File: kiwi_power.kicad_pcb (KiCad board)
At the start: 2 copper layers, 100 x 92 mm, 60 parts, among them J1 PSU, J10 Power_output, J2 Battery, J3 emergency_stop, J4 Power_always, J5 Power_stop, J6 Power_output, J7 Power_output, J8 Power_output, J9 Power_output, K1 SANYOU_SRD_Form_C, Q1 BC327, Q2 IRF9540N, Q3 BC327, Q4 BC327, Q5 IRF9540N, Q6 BC327, U1 LM317_TO-220, U2 lm2596_blue_board, U3 lm2596_blue_board, U4 lm2596_blue_board, U5 lm2596_blue_board, U6 lm2596_blue_board

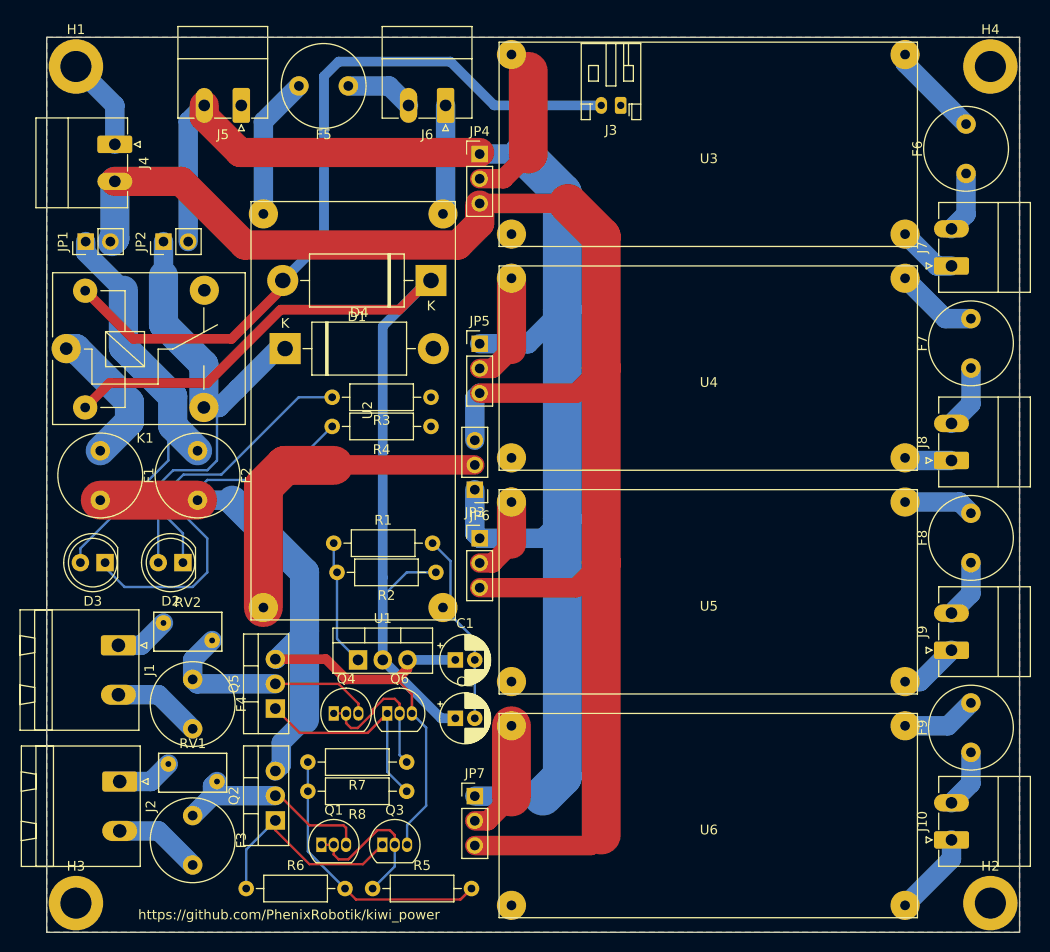
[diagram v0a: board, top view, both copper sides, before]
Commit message: version 2
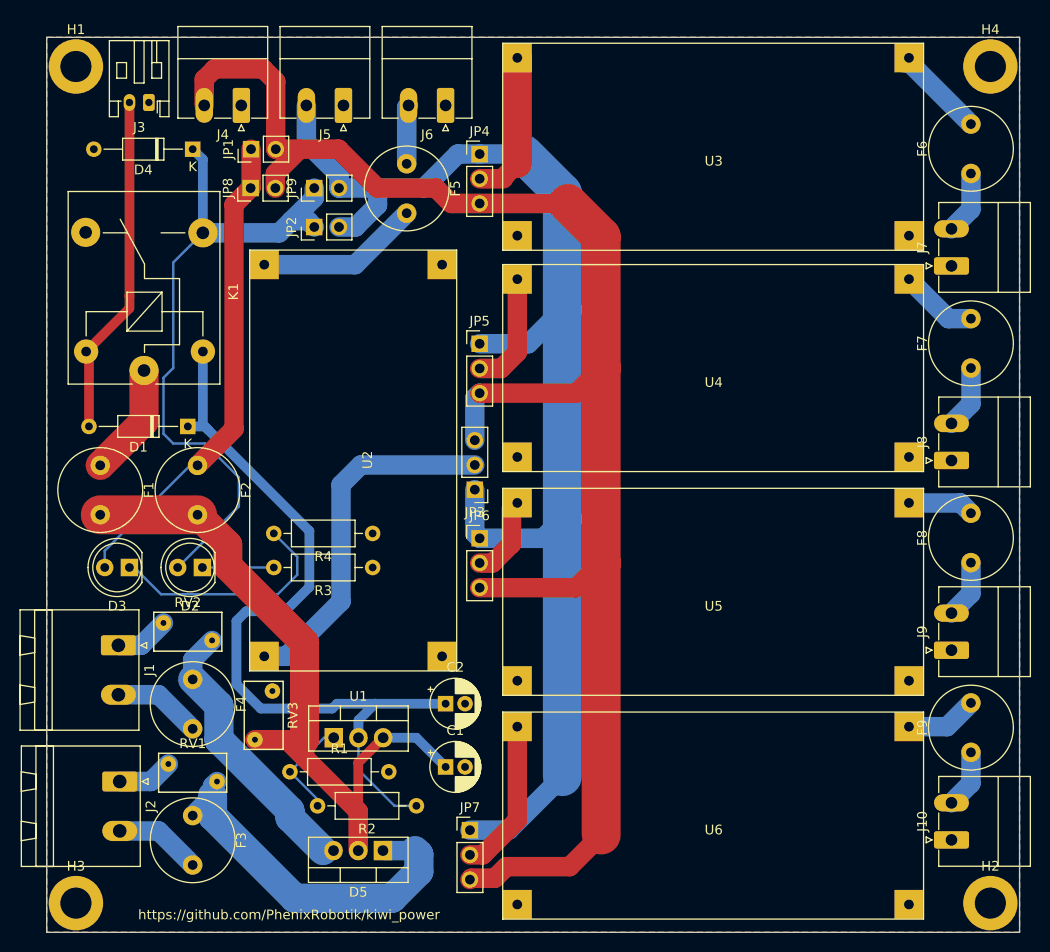
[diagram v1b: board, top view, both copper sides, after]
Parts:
- removed G***: LOGO, kiwi_power:pcb_logo
- removed Q1, Q3, Q4, Q6: BC327, Package_TO_SOT_THT:TO-92_Inline
- removed Q2, Q5: IRF9540N, Package_TO_SOT_THT:TO-220-3_Vertical
- removed R5, R6, R7, R8: R, Resistor_THT:R_Axial_DIN0207_L6.3mm_D2.5mm_P10.16mm_Horizontal
- added D5: C3D16060D, Package_TO_SOT_THT:TO-220-3_Vertical, F.Cu at (214.6, 103.6)
- added JP8: Jumper_NO_Small, Connector_PinHeader_2.54mm:PinHeader_1x02_P2.54mm_Vertical, F.Cu at (201.0, 35.5)
- added JP9: Jumper_NO_Small, Connector_PinHeader_2.54mm:PinHeader_1x02_P2.54mm_Vertical, F.Cu at (207.5, 35.5)
- added RV3: Varistor, Varistor:RV_Disc_D7mm_W4mm_P5mm, F.Cu at (201.4, 92.2)
- D1, D4: footprint Diode_THT:D_DO-201AD_P15.24mm_Horizontal -> Diode_THT:D_DO-35_SOD27_P10.16mm_Horizontal
- moved J3 48.5 mm to (190.5, 26.7)
- moved D1 29.2 mm to (194.5, 60.0)
- moved R2 24.1 mm to (218.0, 99.0)
- moved R1 23.9 mm to (205.0, 95.5)
- moved D4 22.6 mm to (195.0, 31.5), turned to 180 degrees
- moved JP1 19.5 mm to (201.0, 31.5)
- moved R3 18.5 mm to (213.5, 74.5)
- moved JP2 15.6 mm to (207.5, 39.5)
- moved J4 13.6 mm to (200.0, 27.0), turned to 180 degrees
- moved R4 12.5 mm to (213.5, 71.0)
- moved C1 11.0 mm to (221.0, 95.0)
- moved J5 10.5 mm to (210.5, 27.0)
- moved F5 10.0 mm to (217.0, 33.0), turned to 270 degrees
- moved U1 8.38 mm to (209.5, 92.0)
- moved K1 8.31 mm to (190.0, 54.2), turned to 90 degrees
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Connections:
- net Net-(F4-Pad1) renamed /power_input/sheet61577D25/Vout+
- C1 pad 1: /power_input/input_bloc/Vout+ -> Net-(C1-Pad1)
- F1 pad 2: /power_input/input_bloc/Vout+ -> Net-(C1-Pad1)
- F2 pad 2: /power_input/input_bloc/Vout+ -> Net-(C1-Pad1)
- F3 pad 1: Net-(F3-Pad1) -> /power_input/input_bloc/Vout+
- RV1 pad 1: Net-(F3-Pad1) -> /power_input/input_bloc/Vout+
- U1 pad 3: /power_input/input_bloc/Vout+ -> Net-(C1-Pad1)
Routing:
- net GND: track 107.0 -> 11.3 mm
- net Net-(C1-Pad1): track 0.00 -> 77.5 mm
- net /power_input/input_bloc/Vout+: track 89.7 -> 38.0 mm
- net /power_input/emergency_stop: track 79.4 -> 35.3 mm
- net Net-(Q2-Pad1): track 22.5 -> 0.00 mm
- net Net-(Q5-Pad1): track 22.2 -> 0.00 mm
- net Net-(D2-Pad1): track 28.9 -> 7.34 mm
- net Net-(F3-Pad1): track 21.4 -> 0.00 mm
- net /power_input/V_power_stop: track 52.2 -> 69.4 mm
- net Net-(Q1-Pad1): track 16.6 -> 0.00 mm
- net Net-(D3-Pad1): track 40.4 -> 24.5 mm
- net Net-(Q4-Pad1): track 15.9 -> 0.00 mm
- net Net-(C2-Pad1): track 98.1 -> 84.7 mm
- net /regulators/V_in_stop: track 150.1 -> 138.9 mm
- net /power_input/V_power_always: track 44.6 -> 49.7 mm
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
